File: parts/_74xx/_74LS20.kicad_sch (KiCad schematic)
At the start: 2 parts, among them U1 NAND5, U2 NAND5

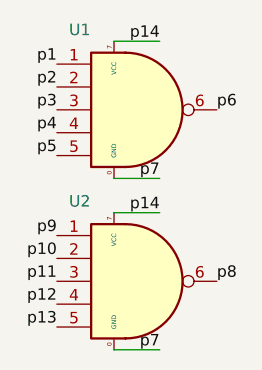
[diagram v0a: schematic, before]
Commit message: Added/Updated parts.
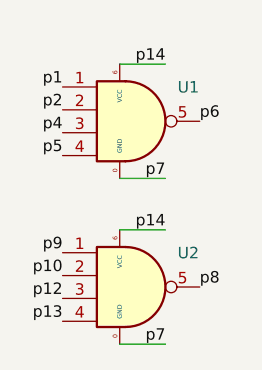
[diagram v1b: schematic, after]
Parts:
- removed U1, U2: NAND5, symbol SimCad:NAND5
- added U1, U2: NAND4, symbol SimCad:NAND4
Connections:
- net p1: now also U1.1
- net p10: now also U2.2
- net p12: now also U2.3
- net p13: now also U2.4
- net p14: now also U1.6 (VCC), U2.6 (VCC)
- net p2: now also U1.2
- net p4: now also U1.3
- net p5: now also U1.4
- net p6: now also U1.5
- net p7: now also U1.0 (GND), U2.0 (GND)
- net p8: now also U2.5
- net p9: now also U2.1
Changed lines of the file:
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@@
 	(wire
 		(pts
-			(xy 157.48 111.76) (xy 162.56 111.76)
+			(xy 158.115 111.125) (xy 163.195 111.125)
 		)
 		(stroke
@@
 	(wire
 		(pts
-			(xy 157.48 77.47) (xy 162.56 77.47)
+			(xy 158.115 80.01) (xy 163.195 80.01)
 		)
 		(stroke
@@
 	(wire
 		(pts
-			(xy 157.48 96.52) (xy 162.56 96.52)
+			(xy 158.115 92.71) (xy 163.195 92.71)
 		)
 		(stroke
@@
 	(wire
 		(pts
-			(xy 157.48 92.71) (xy 162.56 92.71)
+			(xy 158.115 98.425) (xy 163.195 98.425)
 		)
 		(stroke
@@
 		)
 	)
-	(label "p11"
-		(at 151.13 104.14 180)
-		(effects
-			(font
-				(size 1.27 1.27)
-			)
-			(justify right bottom)
-		)
-	)
 	(label "p2"
-		(at 151.13 82.55 180)
+		(at 151.765 85.09 180)
 		(effects
 			(font
@@
 	)
 	(label "p14"
-		(at 162.56 96.52 180)
+		(at 163.195 98.425 180)
 		(effects
 			(font
@@
 	)
 	(label "p7"
-		(at 162.56 92.71 180)
+		(at 163.195 92.71 180)
 		(effects
 			(font
@@
 	)
 	(label "p7"
-		(at 162.56 111.76 180)
+		(at 163.195 111.125 180)
 		(effects
 			(font
@@
 	)
 	(label "p6"
-		(at 168.91 85.09 0)
+		(at 167.005 86.36 0)
 		(effects
 			(font
@@
 	)
 	(label "p4"
-		(at 151.13 87.63 180)
+		(at 151.765 87.63 180)
 		(effects
 			(font
@@
 	)
 	(label "p10"
-		(at 151.13 101.6 180)
-		(effects
-			(font
-				(size 1.27 1.27)
-			)
-			(justify right bottom)
-		)
-	)
-	(label "p3"
-		(at 151.13 85.09 180)
+		(at 151.765 103.505 180)
 		(effects
 			(font
@@
 	)
 	(label "p9"
-		(at 151.13 99.06 180)
+		(at 151.765 100.965 180)
 		(effects
 			(font
@@
 	)
 	(label "p5"
-		(at 151.13 90.17 180)
+		(at 151.765 90.17 180)
 		(effects
 			(font
@@
 	)
 	(label "p14"
-		(at 162.56 77.47 180)
+		(at 163.195 80.01 180)
 		(effects
 			(font
@@
 	)
 	(label "p13"
-		(at 151.13 109.22 180)
+		(at 151.765 108.585 180)
 		(effects
 			(font
@@
 	)
 	(label "p8"
-		(at 168.91 104.14 0)
+		(at 167.005 104.775 0)
 		(effects
 			(font
@@
 	)
 	(label "p12"
-		(at 151.13 106.68 180)
+		(at 151.765 106.045 180)
 		(effects
 			(font
@@
 	)
 	(label "p1"
-		(at 151.13 80.01 180)
+		(at 151.765 82.55 180)
 		(effects
 			(font
@@
 	)
 	(symbol
-		(lib_id "SimCad:NAND5")
-		(at 157.48 85.09 0)
+		(lib_id "SimCad:NAND4")
+		(at 158.115 104.775 0)
 		(unit 1)
 		(exclude_from_sim no)
@@
 		(on_board yes)
 		(dnp no)
+		(fields_autoplaced yes)
+		(property "Reference" "U2"
+			(at 165.735 100.9964 0)
+			(effects
+				(font
+					(size 1.27 1.27)
+				)
+			)
+		)
+		(property "Value" "NAND4"
+			(at 158.115 94.615 0)
+			(effects
+				(font
+					(size 1.27 1.27)
+				)
+				(hide yes)
+			)
+		)
+		(property "Footprint" ""
+			(at 144.145 94.615 0)
+			(effects
+				(font
+					(size 1.27 1.27)
+				)
+				(hide yes)
+			)
+		)
+		(property "Datasheet" ""
+			(at 144.145 94.615 0)
+			(effects
+				(font
+					(size 1.27 1.27)
+				)
+				(hide yes)
+			)
+		)
+		(property "Description" ""
+			(at 158.115 104.775 0)
+			(effects
+				(font
+					(size 1.27 1.27)
+				)
+				(hide yes)
+			)
+		)
+		(pin "6"
+		)
+		(pin "5"
+		)
+		(pin "2"
+		)
+		(pin "3"
+		)
+		(pin "4"
+		)
+		(pin "0"
+		)
+		(pin "1"
+		)
+		(instances
+			(project "_74LS20"
+				(path "/1b0af713-4f45-4868-8c1a-65e627735a28"
+					(reference "U2")
+					(unit 1)
+				)
+			)
+		)
+	)
+	(symbol
+		(lib_id "SimCad:NAND4")
+		(at 158.115 86.36 0)
+		(unit 1)
+		(exclude_from_sim no)
+		(in_bom yes)
+		(on_board yes)
+		(dnp no)
+		(fields_autoplaced yes)
 		(property "Reference" "U1"
-			(at 153.67 76.2 0)
-			(effects
-				(font
-					(size 1.27 1.27)
-				)
-			)
-		)
-		(property "Value" "NAND5"
-			(at 162.56 76.2 0)
+			(at 165.735 82.5814 0)
+			(effects
+				(font
+					(size 1.27 1.27)
+				)
+			)
+		)
+		(property "Value" "NAND4"
+			(at 158.115 76.2 0)
 			(effects
 				(font
@@
 		)
 		(property "Footprint" ""
-			(at 143.51 73.66 0)
+			(at 144.145 76.2 0)
 			(effects
 				(font
@@
 		)
 		(property "Datasheet" ""
-			(at 143.51 73.66 0)
+			(at 144.145 76.2 0)
 			(effects
 				(font
@@
 		)
 		(property "Description" ""
-			(at 157.48 85.09 0)
+			(at 158.115 86.36 0)
 			(effects
 				(font
@@
 		(pin "6"
 		)
+		(pin "5"
+		)
+		(pin "2"
+		)
+		(pin "3"
+		)
+		(pin "4"
+		)
 		(pin "0"
 		)
-		(pin "5"
-		)
-		(pin "3"
-		)
-		(pin "4"
-		)
-		(pin "2"
-		)
 		(pin "1"
-		)
-		(pin "7"
 		)
 		(instances
@@
 					(unit 1)
 				)
-			)
-		)
-	)
-	(symbol
-		(lib_id "SimCad:NAND5")
-		(at 157.48 104.14 0)
-		(unit 1)
-		(exclude_from_sim no)
-		(in_bom yes)
-		(on_board yes)
-		(dnp no)
-		(property "Reference" "U2"
-			(at 153.67 95.25 0)
-			(effects
-				(font
-					(size 1.27 1.27)
-				)
-			)
-		)
-		(property "Value" "NAND5"
-			(at 162.56 95.25 0)
-			(effects
-				(font
-					(size 1.27 1.27)
-				)
-				(hide yes)
-			)
-		)
-		(property "Footprint" ""
-			(at 143.51 92.71 0)
-			(effects
-				(font
-					(size 1.27 1.27)
-				)
-				(hide yes)
-			)
-		)
-		(property "Datasheet" ""
-			(at 143.51 92.71 0)
-			(effects
-				(font
-					(size 1.27 1.27)
-				)
-				(hide yes)
-			)
-		)
-		(property "Description" ""
-			(at 157.48 104.14 0)
-			(effects
-				(font
-					(size 1.27 1.27)
-				)
-				(hide yes)
-			)
-		)
-		(pin "5"
-		)
-		(pin "3"
-		)
-		(pin "4"
-		)
-		(pin "0"
-		)
-		(pin "6"
-		)
-		(pin "7"
-		)
-		(pin "2"
-		)
-		(pin "1"
-		)
-		(instances
-			(project ""
-				(path "/1b0af713-4f45-4868-8c1a-65e627735a28"
-					(reference "U2")
-					(unit 1)
-				)
